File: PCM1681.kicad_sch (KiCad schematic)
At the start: 37 parts, among them J1 USB_C_Receptacle_PowerOnly_6P, J2 Conn_01x10_Pin, J3 Conn_01x05_Pin, J4 Conn_01x05_Pin, J5 Conn_01x05_Pin, J6 AudioJack3, J7 AudioJack3, J8 AudioJack3, J9 AudioJack3, SW1 SW_DIP_x04, U1 AMS1117-3.3, U2 NJW4191M, U3 PCM1681

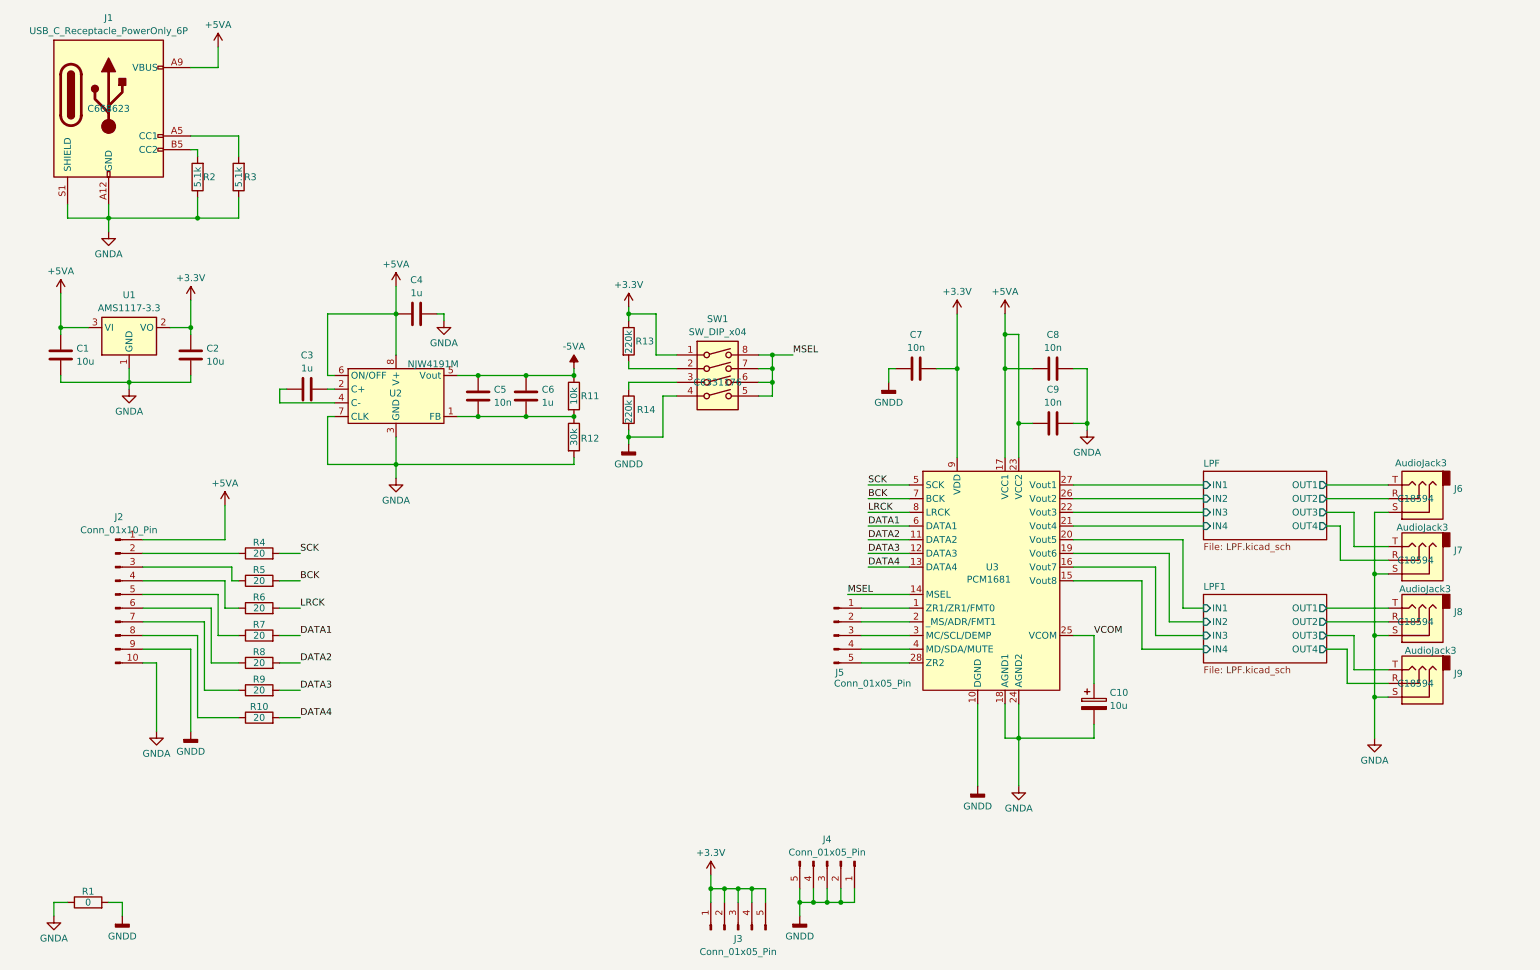
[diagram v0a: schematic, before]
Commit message: First order
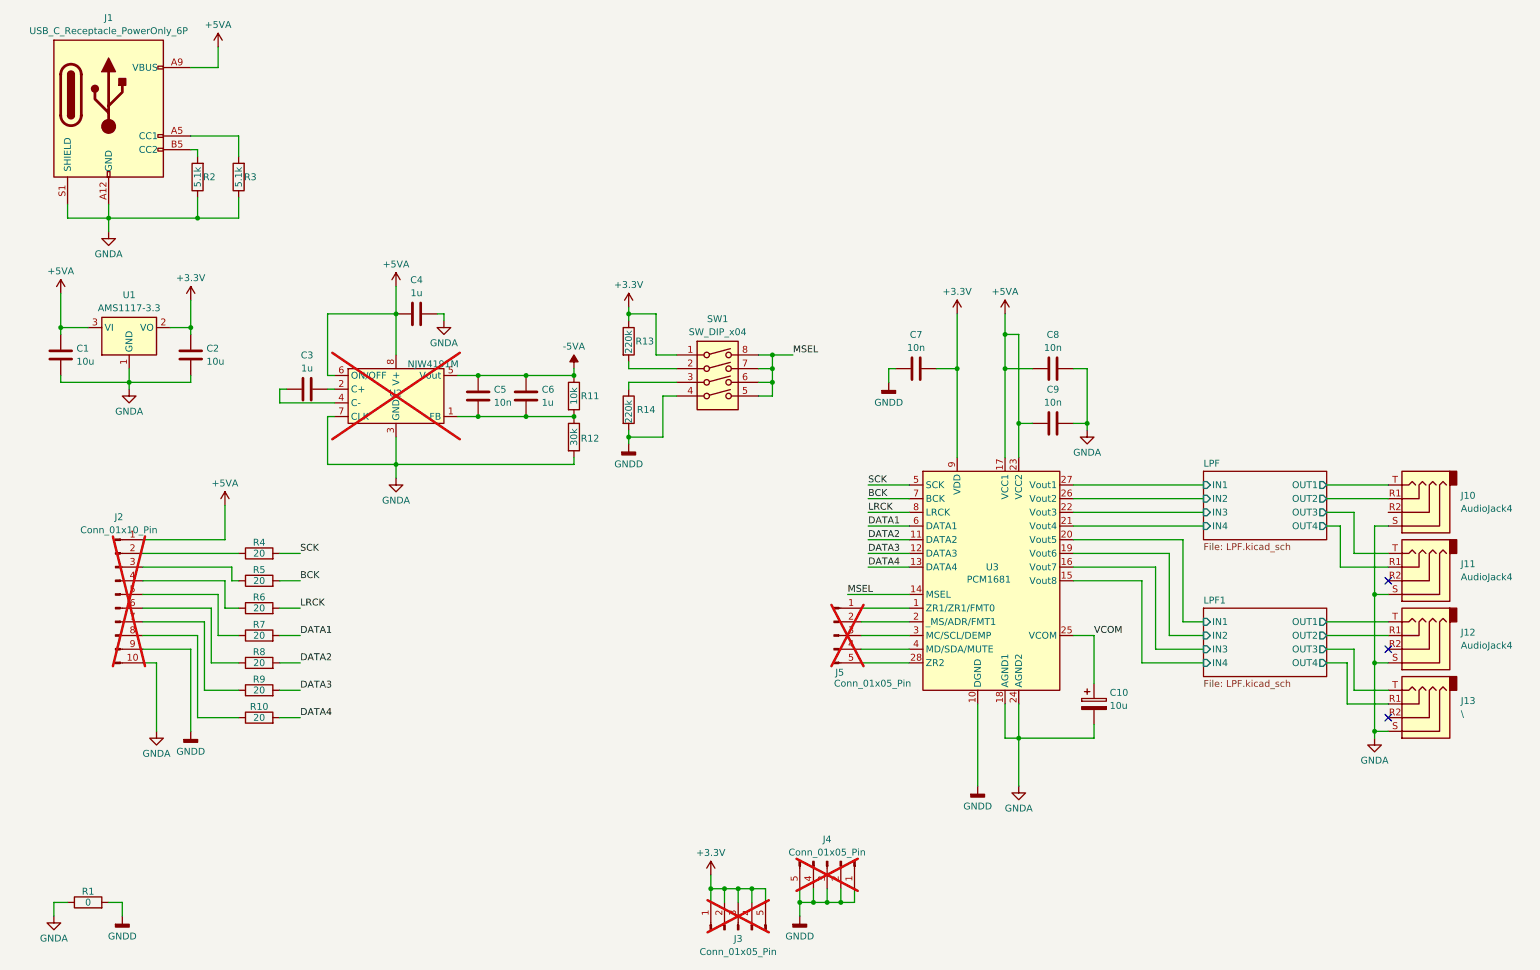
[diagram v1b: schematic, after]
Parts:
- removed J6, J7, J8, J9: AudioJack3, Connector_Audio:Jack_3.5mm_CUI_SJ-3523-SMT_Horizontal, symbol Connector_Audio:AudioJack3
- added J10, J11, J12: AudioJack4, Connector_Audio:Jack_3.5mm_PJ320D_Horizontal, symbol Connector_Audio:AudioJack4
- added J13: \, Connector_Audio:Jack_3.5mm_PJ320D_Horizontal, symbol Connector_Audio:AudioJack4
- C5, C7, C8, C9: LCSC C15195 -> C15195
- J2, J3, J4, J5, U2: now not fitted
- U1: LCSC AMS1117-3.3 C6186 -> C6186
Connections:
- net GNDA: now also J10.S, J11.S, J12.S, J13.S
- net LPF/OUT1: now also J10.T
- net LPF/OUT2: now also J10.R1
- net LPF/OUT3: now also J11.T
- net LPF/OUT4: now also J11.R1
- net LPF1/OUT1: now also J12.T
- net LPF1/OUT2: now also J12.R1
- net LPF1/OUT3: now also J13.T
- net LPF1/OUT4: now also J13.R1
- no-connect marks 0 -> 3
